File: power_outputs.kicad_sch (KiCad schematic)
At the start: 10 parts, among them Q1 BSS138, Q3 MMBT3904, Q4 MMBT3906

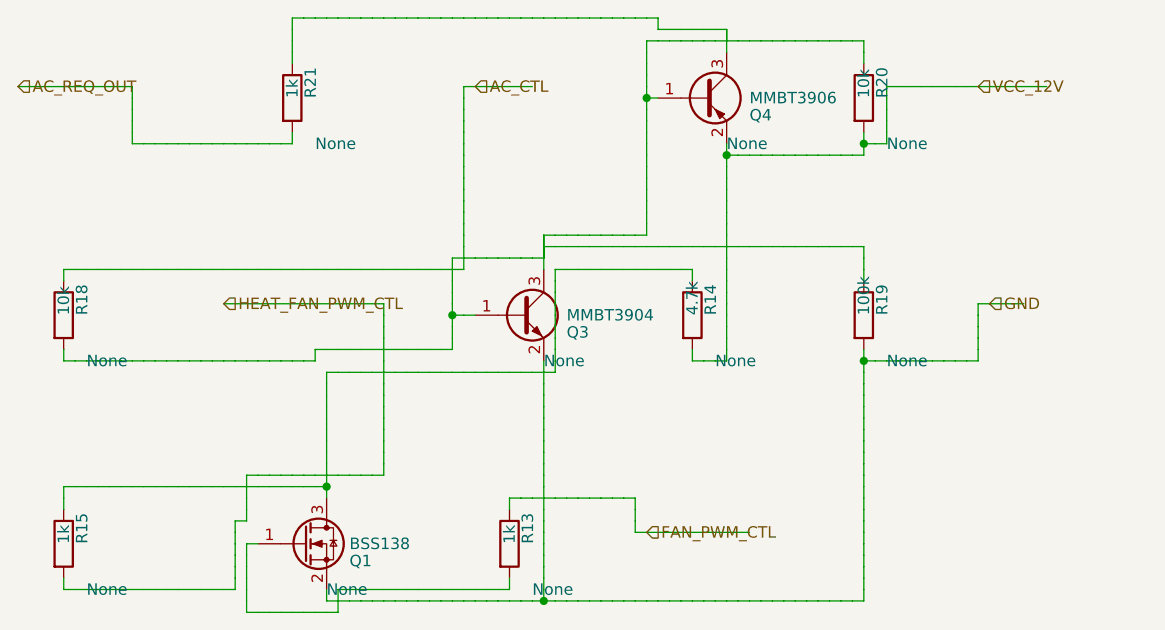
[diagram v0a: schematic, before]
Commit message: fix writer
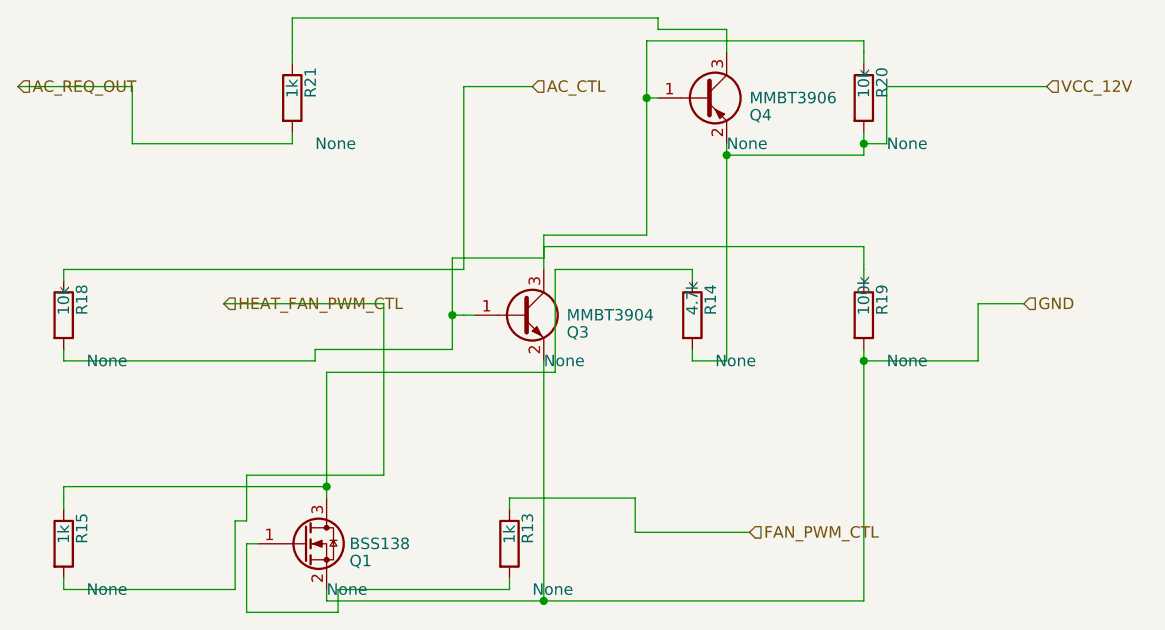
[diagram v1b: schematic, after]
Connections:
- net AC_CTL: no longer Q1.1 (G), Q1.2 (S), Q1.3 (D), Q3.1 (B), Q3.2 (E), Q3.3 (C), Q4.1 (B), Q4.2 (E), Q4.3 (C), R13.1, R13.2, R14.1, R14.2, R15.1, R15.2, R18.2, R19.1, R19.2, R20.1, R20.2, R21.1
- new net: Q1.3 (D), R14.1, R15.1
- new net: Q3.1 (B), Q3.3 (C), Q4.1 (B), R18.2, R19.1, R20.1
- new net: Q4.3 (C), R21.1
- new net: Q1.1 (G), R13.2
- new net FAN_PWM_CTL: R13.1
- new net GND: Q1.2 (S), Q3.2 (E), R19.2
- new net HEAT_FAN_PWM_CTL: R15.2
- new net VCC_12V: Q4.2 (E), R14.2, R20.2
